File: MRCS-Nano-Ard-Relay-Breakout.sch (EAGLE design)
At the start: 9 parts, among them CON1 5V PWR, J1 5V PWR, J2 Unused I/O, J4 Outputs

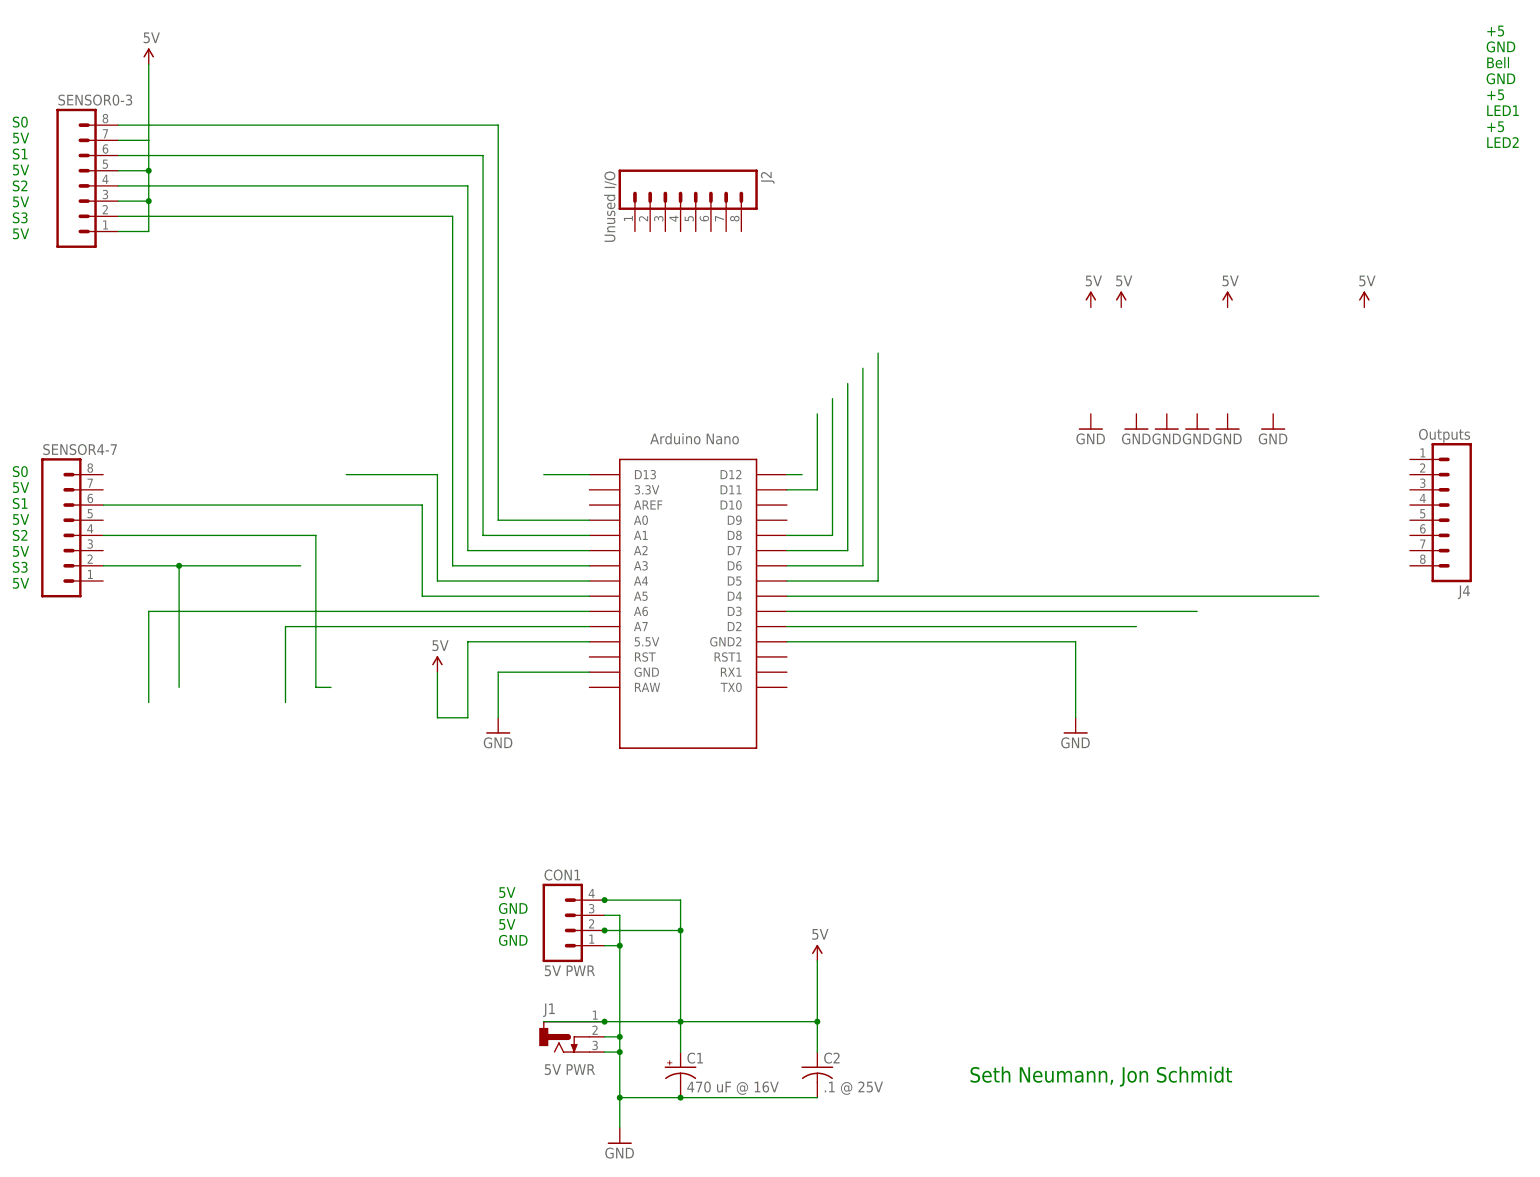
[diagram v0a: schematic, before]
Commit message: files as sent to jlcpcb for 1st run
completion of design
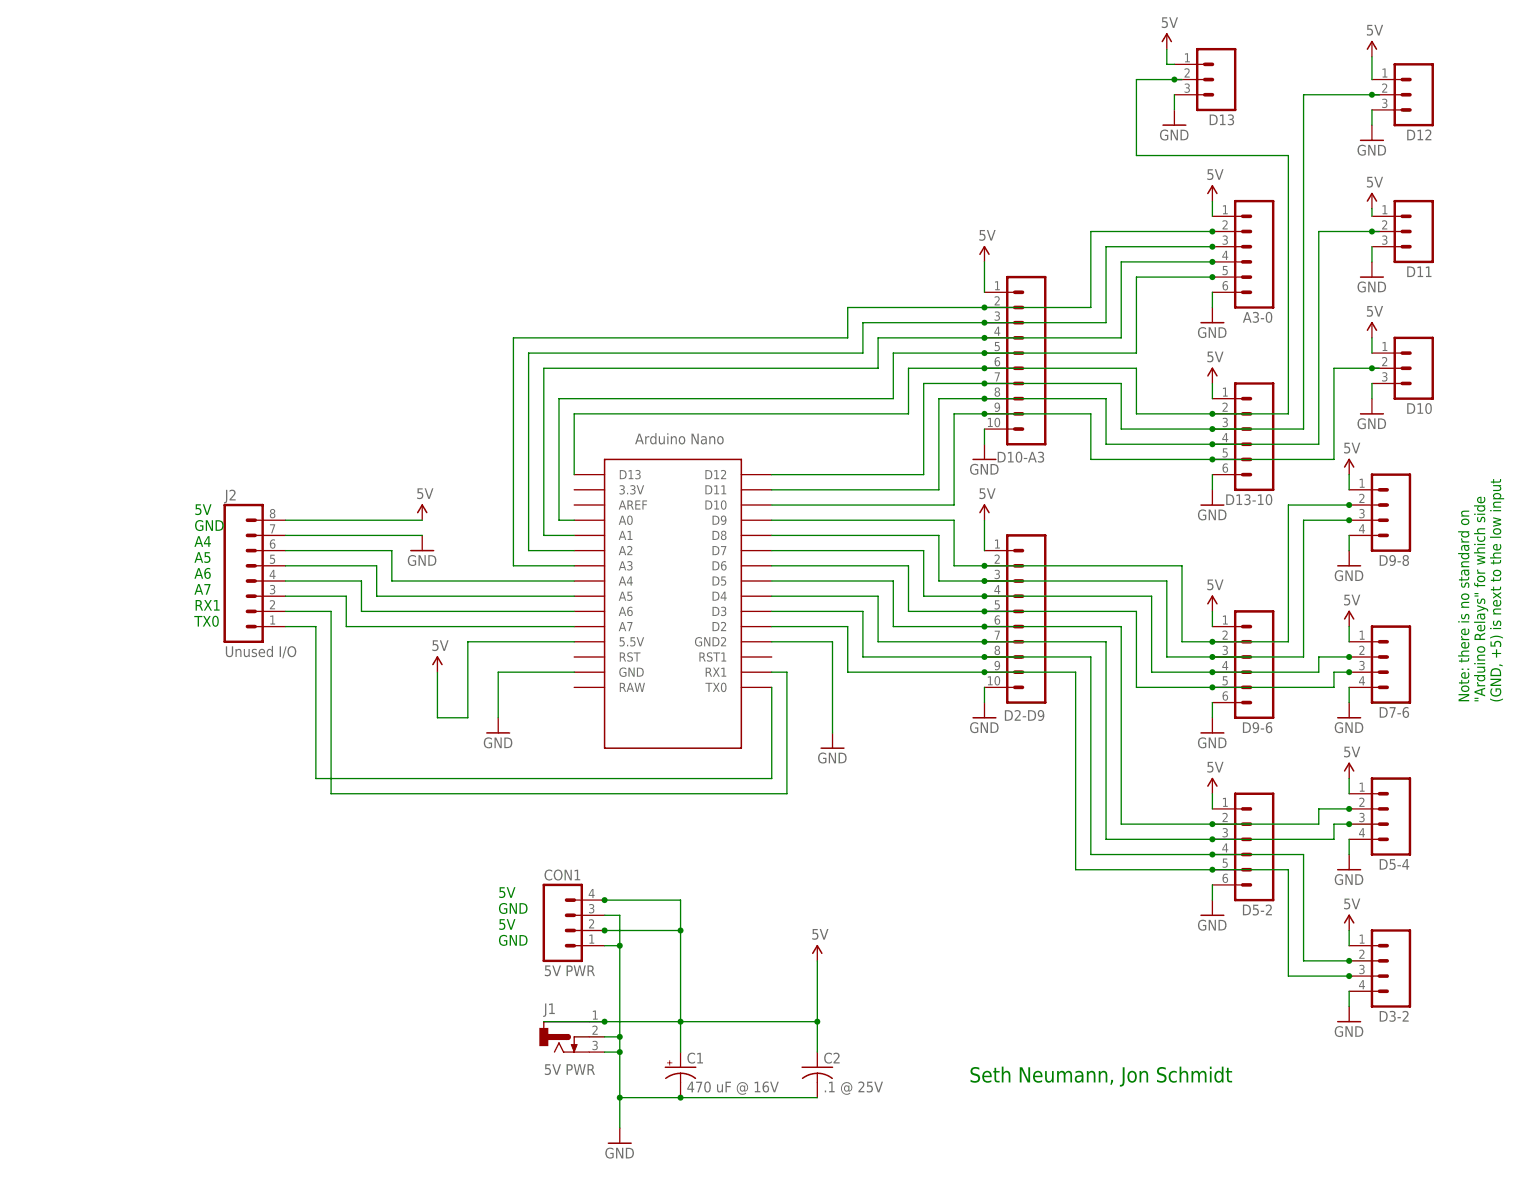
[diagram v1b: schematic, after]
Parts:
- removed J4: Outputs, SPCoast:CONNECTOR-M08LOCK
- removed SENSOR0-3, SENSOR4-7: (no value), SPCoast:CONNECTOR-M08LOCK
- added A3-0, D13-10, D5-2, D9-6: (no value), SPCoast:CONNECTOR-M06LOCK
- added D10, D11, D12, D13: CONNECTOR-M03MOLEX-254-LOCK, SPCoast:CONNECTOR-M03MOLEX-254-LOCK
- added D10-A3, D2-D9: CONNECTOR-M102MM, SPCoast:CONNECTOR-M102MM
- added D3-2, D5-4, D7-6, D9-8: (no value), SPCoast:CONNECTOR-M04LOCK
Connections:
- removed net A0: SENSOR0-3.8, U$1.A0
- removed net N$1: U$1.A4
- removed net N$2: U$1.D2
- removed net N$20: U$1.D12
- removed net N$21: U$1.D11
- removed net N$22: U$1.D8
- removed net N$24: U$1.D6
- removed net N$25: U$1.D5
- removed net N$6: U$1.D4
- new net A4: J2.6, U$1.A4
- new net A5: J2.5, U$1.A5
- new net A6: J2.4, U$1.A6
- new net A7: J2.3, U$1.A7
- new net N$14: D10-A3.6, D13-10.2, D13.2, U$1.D13
- new net N$18: A3-0.2, D10-A3.2, U$1.A3
- new net N$19: D2-D9.7, D5-2.3, D5-4.3, U$1.D4
- new net N$8: D2-D9.4, D7-6.2, D9-6.4, U$1.D7
- new net N$9: D2-D9.3, D9-6.3, D9-8.3, U$1.D8
- new net RX1: J2.2, U$1.RX1
- new net TX0: J2.1, U$1.TX0
- net 5V: now also A3-0.1, D10-A3.1, D10.1, D11.1, D12.1, D13-10.1, D13.1, D2-D9.1, D3-2.1, D5-2.1, D5-4.1, D7-6.1, D9-6.1, D9-8.1, J2.8; no longer SENSOR0-3.1, SENSOR0-3.3, SENSOR0-3.5, SENSOR0-3.7
- net GND: now also A3-0.6, D10-A3.10, D10.3, D11.3, D12.3, D13-10.6, D13.3, D2-D9.10, D3-2.4, D5-2.6, D5-4.4, D7-6.4, D9-6.6, D9-8.4, J2.7
- net N$10: now also D2-D9.2, D9-6.2, D9-8.2, U$1.D9; no longer SENSOR0-3.4, U$1.A2
- net N$11: now also D10-A3.9, D10.2, D13-10.5, U$1.D10; no longer SENSOR4-7.4
- net N$12: now also D10-A3.8, D11.2, D13-10.4, U$1.D11; no longer SENSOR0-3.2, U$1.A3
- net N$13: now also D10-A3.7, D12.2, D13-10.3, U$1.D12; no longer SENSOR4-7.2
- net N$15: now also A3-0.5, D10-A3.5, U$1.A0; no longer U$1.A6
- net N$16: now also A3-0.4, D10-A3.4, U$1.A1; no longer U$1.A7
- net N$17: now also A3-0.3, D10-A3.3, U$1.A2; no longer SENSOR0-3.6, U$1.A1
- net N$23: now also D2-D9.6, D5-2.2, D5-4.2, U$1.D5; no longer U$1.D7
- net N$3: now also D2-D9.9, D3-2.3, D5-2.5, U$1.D2; no longer U$1.D13
- net N$4: now also D2-D9.8, D3-2.2, D5-2.4
- net N$7: now also D2-D9.5, D7-6.3, D9-6.5, U$1.D6; no longer SENSOR4-7.6, U$1.A5
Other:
- note added: "5V GND A4 A5 A6 A7 RX1 TX0"
- note added: "Note: there is no standard on "Arduino Relays" for which side (GND, +5) is next to the low input"
- note removed: "+5 GND Bell GND +5 LED1 +5 LED2"
- note removed: "S0 5V S1 5V S2 5V S3 5V"
- moved on the sheet: J2
